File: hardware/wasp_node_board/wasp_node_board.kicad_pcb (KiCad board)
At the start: 4 copper layers, 63.5 x 82.5 mm, 115 parts, among them J1 Conn_01x02, J2 RJ45_Hanrun_HR911105A_Horizon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, J3 Conn_02x10_Odd_Even, J4 RJ45_Hanrun_HR911105A_Horizon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, J5 RJ45_Hanrun_HR911105A_Horizon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, J6 TC2030, J7 USB_C_Receptacle_USB2.0_16P, SW1 C&K JS102011SAQN, SW2 C&K KMR231NG LFS, U1 STM32H723ZGTx, U2 USBLC6-2SC6, U3 APS6404L-3SQRx-SN, U4 TPSM863253RDXR, U5 KSZ8794CNXCC, U6 LP5907MFX-1.2, Y1 TSX-3225 25.00M-N0YYYYG30RGB, Y2 ASE-25.000MHZ-L-K-T

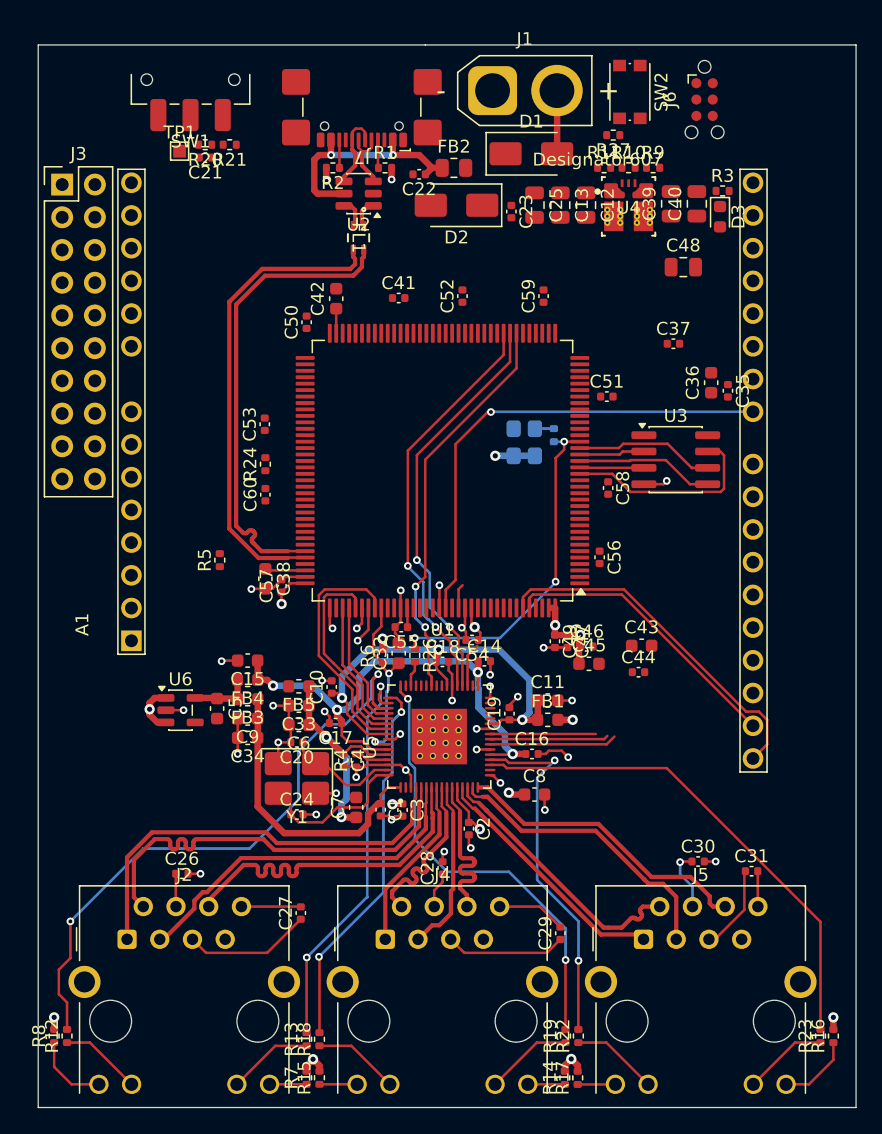
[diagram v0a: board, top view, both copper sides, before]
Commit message: Removed some stuff and got the general placement down
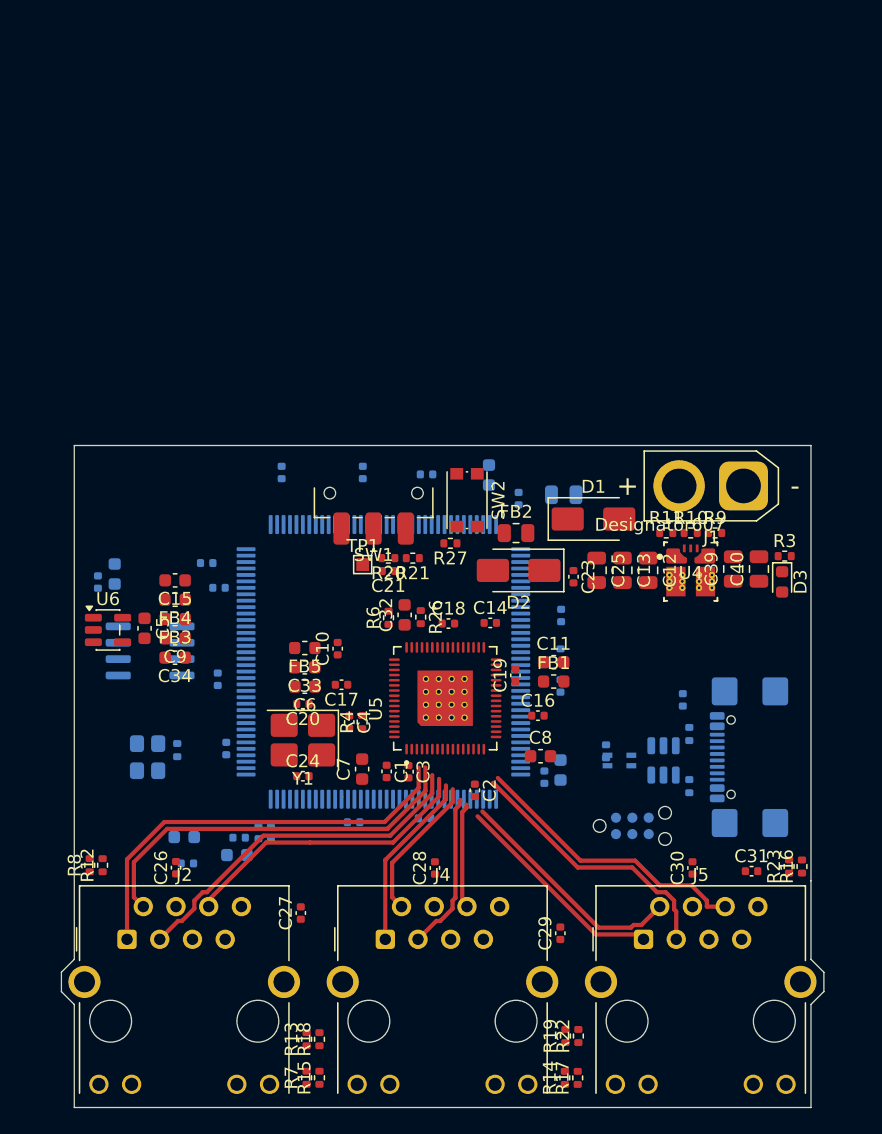
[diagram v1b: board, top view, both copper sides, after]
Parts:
- removed A1: Arduino_UNO_R3, Arduino_UNO_R3_Headers:Arduino_UNO_R3_Headers
- removed J3: Conn_02x10_Odd_Even, Connector_PinHeader_2.54mm:PinHeader_2x10_P2.54mm_Vertical
- C22, C35, C36, C37, C38, C41, C42, C43, C44, C45, C46, C47, C48, C49, C50, C51, C52, C53, C54, C55, C56, C57, C58, C59, C60, FL1, J6, J7, R1, R2, R24, R5, U1, U2, U3: moved to B.Cu
- moved J7 60.3 mm to (158.4, 98.8), turned to -90 degrees
- moved J6 56.7 mm to (148.1, 104.1), turned to 0 degrees
- moved R2 55.4 mm to (152.6, 101.0), turned to -90 degrees
- moved C35 51.1 mm to (106.6, 85.2)
- moved U2 50.0 mm to (150.6, 99.0), turned to -90 degrees
- moved R1 49.9 mm to (152.6, 97.0), turned to 90 degrees
- moved C36 48.6 mm to (107.9, 84.6)
- moved C22 45.7 mm to (152.1, 94.3), turned to -90 degrees
- moved FL1 45.4 mm to (147.1, 99.1), turned to 180 degrees
- moved U3 43.4 mm to (110.7, 90.5), turned to 180 degrees
- moved C37 40.0 mm to (115.1, 83.7), turned to 180 degrees
- moved C43 38.5 mm to (113.3, 105.0), turned to 180 degrees
- moved Y2 38.1 mm to (110.5, 98.8)
- moved R25 38.1 mm to (112.8, 98.2)
- moved C44 38.0 mm to (113.6, 107.0), turned to 180 degrees
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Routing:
- net GND: track 75.2 -> 0.07 mm, vias 34 -> 0
- net Net-(U5-LED1_0): track 49.0 -> 0.00 mm, vias 2 -> 0
- net VDD12D: track 41.6 -> 0.00 mm, vias 4 -> 0
- net VDDAT: track 40.8 -> 0.00 mm, vias 5 -> 0
- net Net-(U5-LED3_1): track 39.1 -> 0.00 mm
- net /mcu/PG12: track 37.2 -> 0.00 mm, vias 1 -> 0
- net USB_D_P: track 36.6 -> 0.00 mm
- net USB_D_N: track 36.6 -> 0.00 mm
- net VDDIO: track 36.3 -> 0.00 mm, vias 3 -> 0
- net Net-(U5-LED2_1): track 34.8 -> 0.00 mm, vias 2 -> 0
- net ETH_RXD1: track 32.1 -> 0.00 mm, vias 2 -> 0
- net ETH_RXD0: track 31.8 -> 0.00 mm, vias 2 -> 0
- net Net-(U5-LED1_1): track 31.2 -> 0.00 mm, vias 2 -> 0
- net ETH_CRS_DV: track 31.2 -> 0.00 mm, vias 2 -> 0
- net +3V3: track 29.5 -> 0.00 mm, vias 12 -> 0
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- removed copper zone on In2.Cu, net +3V3
- removed copper zone on In1.Cu, net GND
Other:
- board size 63.5 x 82.5 mm -> 59.2 x 51.4 mm
